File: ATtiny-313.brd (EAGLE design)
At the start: 22.5 x 60.3 mm, 17 parts, among them IC1 REG1117, IC2 ATtiny85

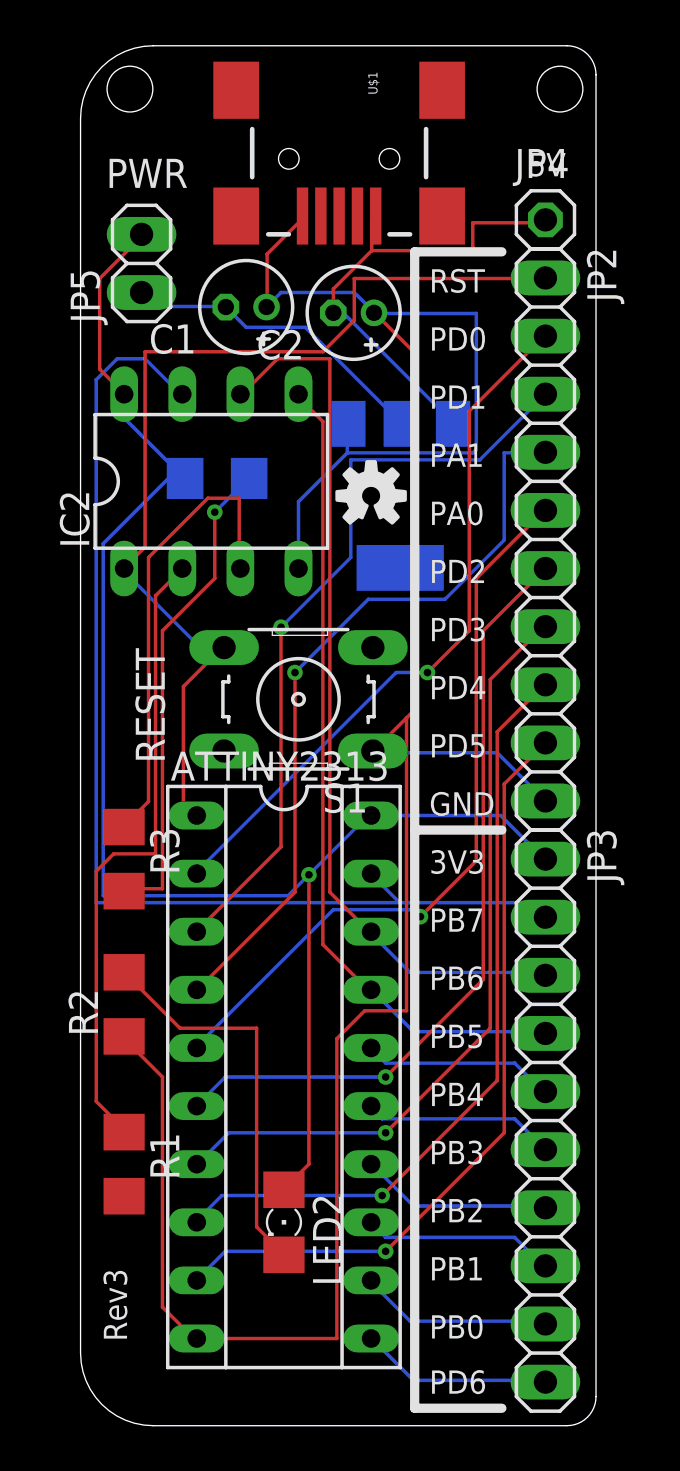
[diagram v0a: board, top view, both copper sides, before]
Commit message: more SMD goodness
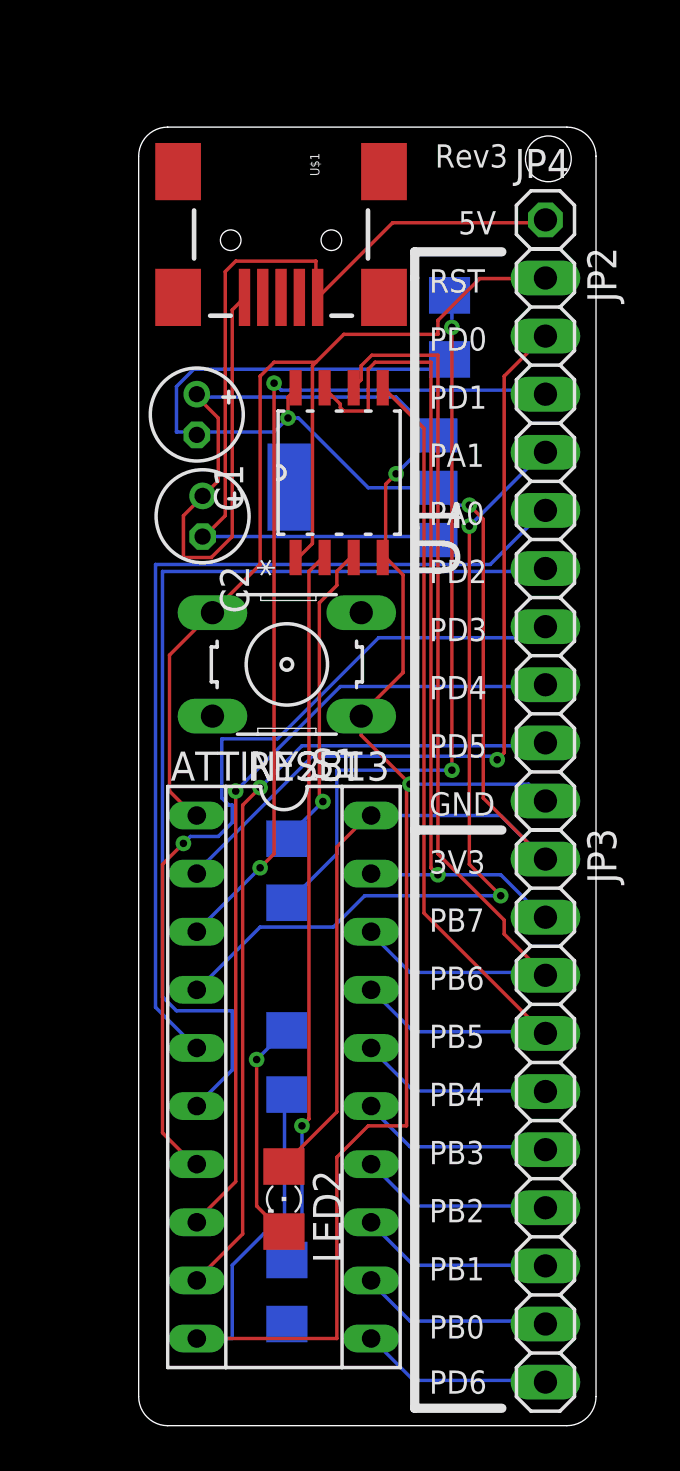
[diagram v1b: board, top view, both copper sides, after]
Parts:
- removed IC2: ATtiny85, ic-package:DIL08
- removed JP5: (no value), pinhead:1X02
- removed U$3: (no value), SparkFun-Aesthetics:OSHW-LOGO-S
- added U1: ATTINY85-20SU, Atmel_By_element14_Batch_1:SOIC127P798X216-8N
- moved R4 12.1 mm to (33.3, 55.6), turned to 270 degrees
- moved C2 11.1 mm to (22.5, 47.4), turned to 270 degrees
- moved R1 9.04 mm to (26.2, 13.5), flipped to the bottom
- moved R2 7.55 mm to (26.2, 23.5), flipped to the bottom
- moved R3 7.13 mm to (26.2, 31.9), flipped to the bottom
- moved C1 5.17 mm to (22.2, 51.8), turned to 270 degrees
- moved U$1 4.37 mm to (25.9, 59.4)
- moved IC1 1.69 mm to (29.5, 48.6), turned to 270 degrees
- moved S1 1.61 mm to (26.2, 40.9)
- moved LED2 1.02 mm to (26.0, 17.5)
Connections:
- removed net N$1: IC2.2, R1.1
- removed net N$2: IC2.3, R3.1
- removed net N$3: C1.-, IC1.2, JP5.1
- new net N$15: R3.1, U1.3
- new net N$16: R1.1, U1.2
- net 3.3V: now also C1.-, IC1.2, U1.8; no longer IC2.8, JP5.2
- net GND: now also U1.4; no longer IC2.4
- net MISO': now also U1.6; no longer IC2.6
- net MOSI': now also U1.5; no longer IC2.5
- net REST': now also U1.1; no longer IC2.1
- net SCLK': now also U1.7; no longer IC2.7
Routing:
- net N$16: track 0.00 -> 31.8 mm, vias 0 -> 1
- net N$1: track 27.8 -> 0.00 mm
- net N$2: track 20.4 -> 0.00 mm
- net 5V: track 21.0 -> 39.4 mm
- net N$3: track 13.7 -> 0.00 mm
- net N$15: track 0.00 -> 13.7 mm, vias 0 -> 1
- net D-': track 21.3 -> 32.6 mm, vias 1 -> 2
- net SCLK': track 49.3 -> 38.1 mm, vias 0 -> 1
- net N$10: track 33.9 -> 43.5 mm, vias 1 -> 0
- net GND: track 112.8 -> 103.8 mm, vias 0 -> 2
- net N$9: track 32.5 -> 39.9 mm, vias 1 -> 0
- net N$24: track 17.2 -> 9.89 mm, vias 0 -> 1
- net N$7: track 33.1 -> 37.4 mm, vias 1 -> 2
- net N$6: track 30.6 -> 34.8 mm
- net N$11: track 33.9 -> 37.7 mm
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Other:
- board size 22.5 x 60.3 mm -> 20 x 56.8 mm
- board text removed: "PWR"
